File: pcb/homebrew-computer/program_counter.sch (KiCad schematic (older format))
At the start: 4 parts, among them U8 XC9536XL-10VQG44C

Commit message: Start working on the pcb layout
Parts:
- C13, C14, C15: footprint (none) -> Capacitor_SMD:C_0402_1005Metric_Pad0.74x0.62mm_HandSolder
- U8: footprint (none) -> Package_QFP:VQFP-44; symbol XC9500XL:XC9536XL-10VQG44C -> homebrew-computer-rescue:XC9536XL-10VQG44C-XC9500XL
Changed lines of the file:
@@
 $Descr User 5906 8268
 encoding utf-8
-Sheet 6 7
+Sheet 7 7
 Title "Program Counter"
 Date "2020-10-26"
@@
 F 0 "C13" H 2392 1696 50  0000 L CNN
 F 1 "100n" H 2392 1605 50  0000 L CNN
-F 2 "" H 2300 1650 50  0001 C CNN
+F 2 "Capacitor_SMD:C_0402_1005Metric_Pad0.74x0.62mm_HandSolder" H 2300 1650 50  0001 C CNN
 F 3 "~" H 2300 1650 50  0001 C CNN
 	1    2300 1650
@@
 F 0 "C14" H 2742 1696 50  0000 L CNN
 F 1 "100n" H 2742 1605 50  0000 L CNN
-F 2 "" H 2650 1650 50  0001 C CNN
+F 2 "Capacitor_SMD:C_0402_1005Metric_Pad0.74x0.62mm_HandSolder" H 2650 1650 50  0001 C CNN
 F 3 "~" H 2650 1650 50  0001 C CNN
 	1    2650 1650
@@
 F 0 "C15" H 3092 1696 50  0000 L CNN
 F 1 "100n" H 3092 1605 50  0000 L CNN
-F 2 "" H 3000 1650 50  0001 C CNN
+F 2 "Capacitor_SMD:C_0402_1005Metric_Pad0.74x0.62mm_HandSolder" H 3000 1650 50  0001 C CNN
 F 3 "~" H 3000 1650 50  0001 C CNN
 	1    3000 1650
@@
 Text HLabel 2850 5250 0    50   Input ~ 0
 TMS
-Text HLabel 2850 5350 0    50   Output ~ 0
-TDO
-Text HLabel 2850 5450 0    50   Input ~ 0
-TDI
 Text HLabel 2850 5550 0    50   Input ~ 0
 TCK
@@
 Inputs/Outputs
 $Comp
-L XC9500XL:XC9536XL-10VQG44C U8
+L homebrew-computer-rescue:XC9536XL-10VQG44C-XC9500XL U8
 U 1 1 5FA8CEAA
 P 3050 5750
+AR Path="/5FA8CEAA" Ref="U8"  Part="1"
+AR Path="/5FA796BE/5FA8CEAA" Ref="U8"  Part="1"
 F 0 "U8" H 2872 5354 50  0000 R CNN
 F 1 "XC9536XL-10VQG44C" H 2872 5445 50  0000 R CNN
-F 2 "" H 3050 5750 50  0001 C CNN
+F 2 "Package_QFP:VQFP-44" H 3050 5750 50  0001 C CNN
 F 3 "" H 3050 5750 50  0001 C CNN
 	1    3050 5750
@@
 $EndComp
 $Comp
-L XC9500XL:XC9536XL-10VQG44C U8
+L homebrew-computer-rescue:XC9536XL-10VQG44C-XC9500XL U8
 U 2 1 5FA9060B
 P 2700 1050
+AR Path="/5FA9060B" Ref="U8"  Part="2"
+AR Path="/5FA796BE/5FA9060B" Ref="U8"  Part="2"
 F 0 "U8" H 2675 1115 50  0000 C CNN
 F 1 "XC9536XL-10VQG44C" H 2675 1024 50  0000 C CNN
-F 2 "" H 2700 1050 50  0001 C CNN
+F 2 "Package_QFP:VQFP-44" H 2700 1050 50  0001 C CNN
 F 3 "" H 2700 1050 50  0001 C CNN
 	2    2700 1050
@@
 Connection ~ 3400 1350
 $Comp
-L XC9500XL:XC9536XL-10VQG44C U8
+L homebrew-computer-rescue:XC9536XL-10VQG44C-XC9500XL U8
 U 3 1 5FA92D8C
 P 3450 1300
+AR Path="/5FA92D8C" Ref="U8"  Part="3"
+AR Path="/5FA796BE/5FA92D8C" Ref="U8"  Part="3"
 F 0 "U8" V 3900 1050 50  0000 R CNN
 F 1 "XC9536XL-10VQG44C" V 3750 1400 50  0000 R CNN
-F 2 "" H 3450 1300 50  0001 C CNN
+F 2 "Package_QFP:VQFP-44" H 3450 1300 50  0001 C CNN
 F 3 "" H 3450 1300 50  0001 C CNN
 	3    3450 1300
@@
 $EndComp
 $Comp
-L XC9500XL:XC9536XL-10VQG44C U8
+L homebrew-computer-rescue:XC9536XL-10VQG44C-XC9500XL U8
 U 5 1 5FA98EFF
 P 3300 2400
+AR Path="/5FA98EFF" Ref="U8"  Part="5"
+AR Path="/5FA796BE/5FA98EFF" Ref="U8"  Part="5"
 F 0 "U8" H 3333 2465 50  0000 C CNN
 F 1 "XC9536XL-10VQG44C" H 3333 2374 50  0000 C CNN
-F 2 "" H 3300 2400 50  0001 C CNN
+F 2 "Package_QFP:VQFP-44" H 3300 2400 50  0001 C CNN
 F 3 "" H 3300 2400 50  0001 C CNN
 	5    3300 2400
@@
 NoConn ~ 2450 4200
 $Comp
-L XC9500XL:XC9536XL-10VQG44C U8
+L homebrew-computer-rescue:XC9536XL-10VQG44C-XC9500XL U8
 U 4 1 5FA96F85
 P 2800 2400
+AR Path="/5FA96F85" Ref="U8"  Part="4"
+AR Path="/5FA796BE/5FA96F85" Ref="U8"  Part="4"
 F 0 "U8" H 2550 400 50  0000 L CNN
 F 1 "XC9536XL-10VQG44C" H 2500 300 50  0000 L CNN
-F 2 "" H 2800 2400 50  0001 C CNN
+F 2 "Package_QFP:VQFP-44" H 2800 2400 50  0001 C CNN
 F 3 "" H 2800 2400 50  0001 C CNN
 	4    2800 2400
@@
 Text GLabel 3600 2600 2    50   3State ~ 0
 BUS1
+Text HLabel 2850 5450 0    50   Input ~ 0
+TDI
+Text HLabel 2850 5350 0    50   Output ~ 0
+TDO
 $EndSCHEMATC

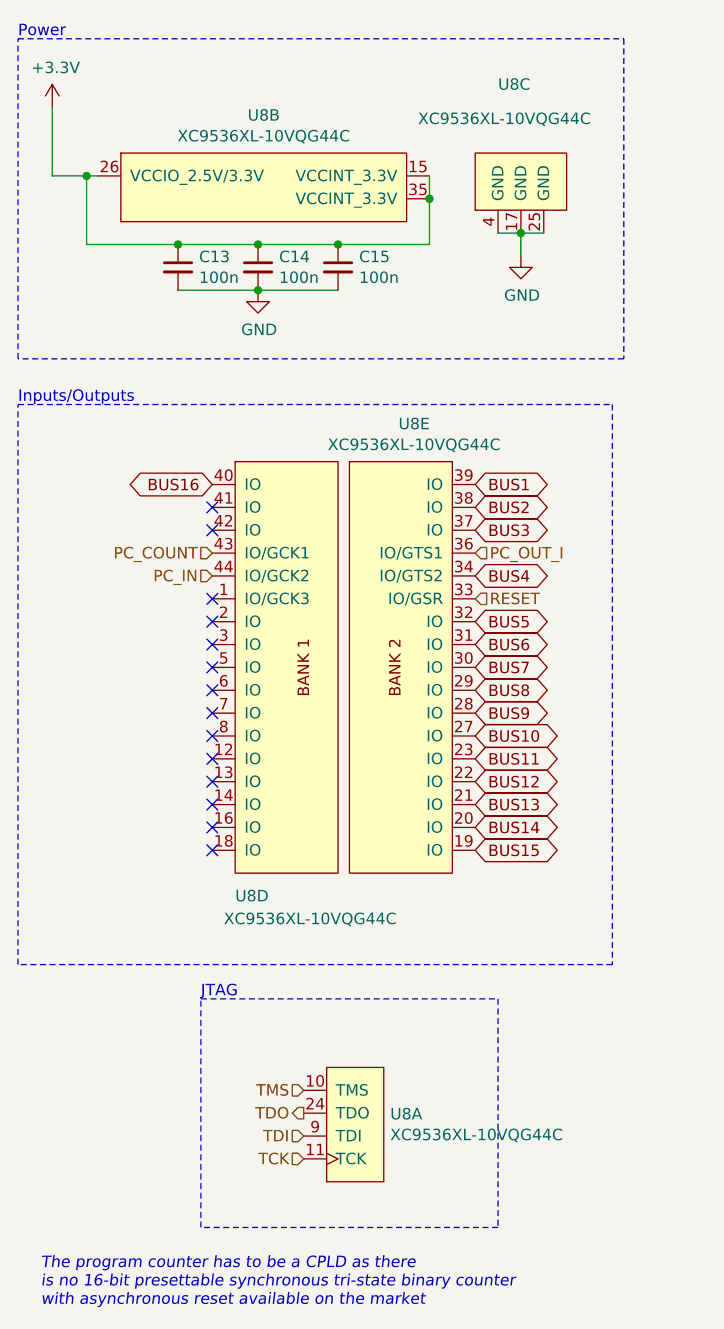
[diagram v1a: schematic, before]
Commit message: Keep working on the layout
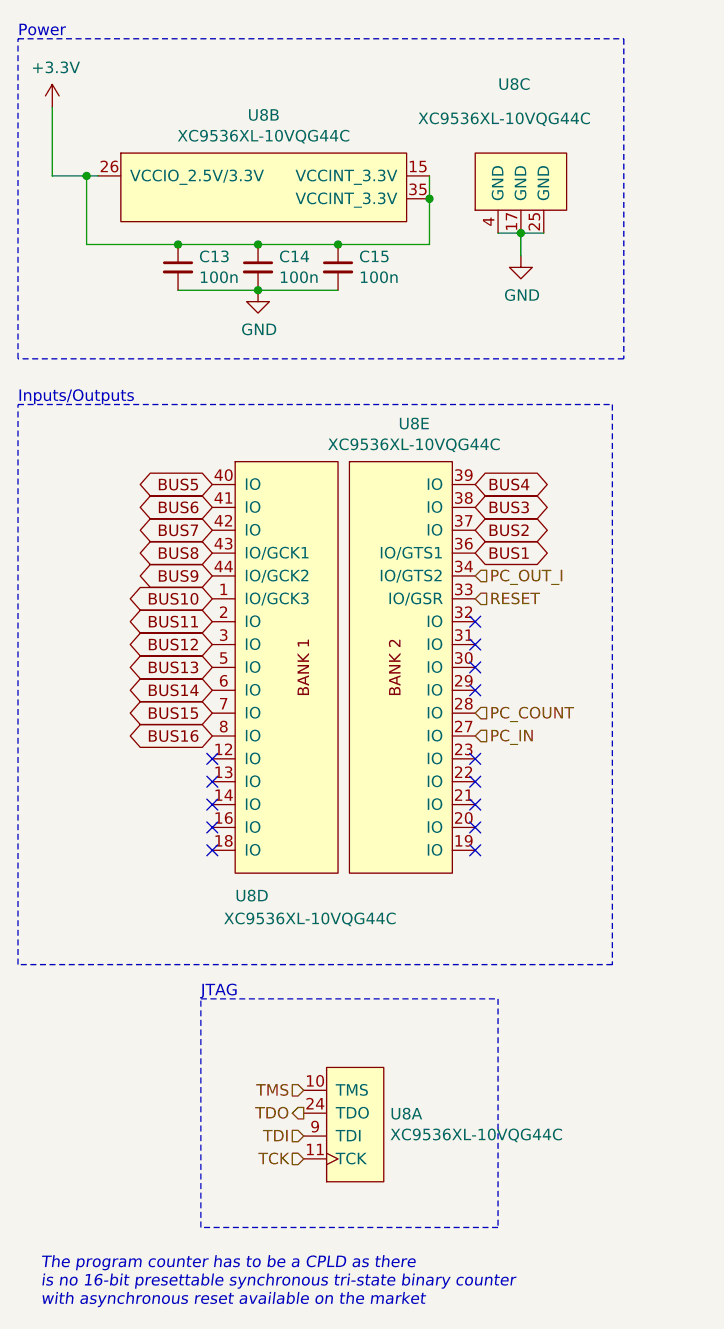
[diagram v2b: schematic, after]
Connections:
- net BUS1: now also U8.36 (IO/GTS1); no longer U8.39 (IO)
- net BUS10: now also U8.1 (IO/GCK3); no longer U8.27 (IO)
- net BUS11: now also U8.2 (IO); no longer U8.23 (IO)
- net BUS12: now also U8.3 (IO); no longer U8.22 (IO)
- net BUS13: now also U8.5 (IO); no longer U8.21 (IO)
- net BUS14: now also U8.6 (IO); no longer U8.20 (IO)
- net BUS15: now also U8.7 (IO); no longer U8.19 (IO)
- net BUS16: now also U8.8 (IO); no longer U8.40 (IO)
- net BUS2: now also U8.37 (IO); no longer U8.38 (IO)
- net BUS3: now also U8.38 (IO); no longer U8.37 (IO)
- net BUS4: now also U8.39 (IO); no longer U8.34 (IO/GTS2)
- net BUS5: now also U8.40 (IO); no longer U8.32 (IO)
- net BUS6: now also U8.41 (IO); no longer U8.31 (IO)
- net BUS7: now also U8.42 (IO); no longer U8.30 (IO)
- net BUS8: now also U8.43 (IO/GCK1); no longer U8.29 (IO)
- net BUS9: now also U8.44 (IO/GCK2); no longer U8.28 (IO)
- net PC_COUNT: now also U8.28 (IO); no longer U8.43 (IO/GCK1)
- net PC_IN: now also U8.27 (IO); no longer U8.44 (IO/GCK2)
- net PC_OUT_I: now also U8.34 (IO/GTS2); no longer U8.36 (IO/GTS1)
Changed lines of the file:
@@
 Text Notes 1700 6200 0    50   Italic 0
 The program counter has to be a CPLD as there\nis no 16-bit presettable synchronous tri-state binary counter\nwith asynchronous reset available on the market
-Text HLabel 2450 2900 0    50   Input ~ 0
+Text HLabel 3600 3600 2    50   Input ~ 0
 PC_COUNT
 Text HLabel 3600 3100 2    50   Input ~ 0
 RESET
-NoConn ~ 2450 2700
-NoConn ~ 2450 2800
-NoConn ~ 2450 3300
-NoConn ~ 2450 3400
-NoConn ~ 2450 3500
-NoConn ~ 2450 3600
-NoConn ~ 2450 3700
-NoConn ~ 2450 3800
-NoConn ~ 2450 3900
-NoConn ~ 2450 4000
-NoConn ~ 2450 4100
-NoConn ~ 2450 4200
+Text HLabel 3600 3700 2    50   Input ~ 0
+PC_IN
+Text HLabel 3600 3000 2    50   Input ~ 0
+PC_OUT_I
+Text GLabel 2450 3600 0    50   3State ~ 0
+BUS15
+Text GLabel 2450 3500 0    50   3State ~ 0
+BUS14
+Text GLabel 2450 3400 0    50   3State ~ 0
+BUS13
+Text GLabel 2450 3300 0    50   3State ~ 0
+BUS12
+Text GLabel 2450 3200 0    50   3State ~ 0
+BUS11
+Text GLabel 2450 3100 0    50   3State ~ 0
+BUS10
+Text GLabel 2450 3000 0    50   3State ~ 0
+BUS9
+Text GLabel 2450 2900 0    50   3State ~ 0
+BUS8
+Text GLabel 2450 2800 0    50   3State ~ 0
+BUS7
+Text GLabel 2450 2700 0    50   3State ~ 0
+BUS6
+Text GLabel 2450 2600 0    50   3State ~ 0
+BUS5
+Text GLabel 3600 2600 2    50   3State ~ 0
+BUS4
+Text GLabel 3600 2700 2    50   3State ~ 0
+BUS3
+Text GLabel 3600 2800 2    50   3State ~ 0
+BUS2
+Text GLabel 3600 2900 2    50   3State ~ 0
+BUS1
+Text HLabel 2850 5450 0    50   Input ~ 0
+TDI
+Text HLabel 2850 5350 0    50   Output ~ 0
+TDO
 $Comp
 L homebrew-computer-rescue:XC9536XL-10VQG44C-XC9500XL U8
@@
 	1    0    0    -1
 $EndComp
-Text HLabel 2450 3000 0    50   Input ~ 0
-PC_IN
-Text HLabel 3600 2900 2    50   Input ~ 0
-PC_OUT_I
-NoConn ~ 2450 3100
-NoConn ~ 2450 3200
-Text GLabel 2450 2600 0    50   3State ~ 0
+Text GLabel 2450 3700 0    50   3State ~ 0
 BUS16
-Text GLabel 3600 4200 2    50   3State ~ 0
-BUS15
-Text GLabel 3600 4100 2    50   3State ~ 0
-BUS14
-Text GLabel 3600 4000 2    50   3State ~ 0
-BUS13
-Text GLabel 3600 3900 2    50   3State ~ 0
-BUS12
-Text GLabel 3600 3800 2    50   3State ~ 0
-BUS11
-Text GLabel 3600 3700 2    50   3State ~ 0
-BUS10
-Text GLabel 3600 3600 2    50   3State ~ 0
-BUS9
-Text GLabel 3600 3500 2    50   3State ~ 0
-BUS8
-Text GLabel 3600 3400 2    50   3State ~ 0
-BUS7
-Text GLabel 3600 3300 2    50   3State ~ 0
-BUS6
-Text GLabel 3600 3200 2    50   3State ~ 0
-BUS5
-Text GLabel 3600 3000 2    50   3State ~ 0
-BUS4
-Text GLabel 3600 2800 2    50   3State ~ 0
-BUS3
-Text GLabel 3600 2700 2    50   3State ~ 0
-BUS2
-Text GLabel 3600 2600 2    50   3State ~ 0
-BUS1
-Text HLabel 2850 5450 0    50   Input ~ 0
-TDI
-Text HLabel 2850 5350 0    50   Output ~ 0
-TDO
+NoConn ~ 2450 3800
+NoConn ~ 2450 3900
+NoConn ~ 2450 4100
+NoConn ~ 2450 4000
+NoConn ~ 2450 4200
+NoConn ~ 3600 4200
+NoConn ~ 3600 4100
+NoConn ~ 3600 4000
+NoConn ~ 3600 3900
+NoConn ~ 3600 3800
+NoConn ~ 3600 3500
+NoConn ~ 3600 3400
+NoConn ~ 3600 3300
+NoConn ~ 3600 3200
 $EndSCHEMATC
